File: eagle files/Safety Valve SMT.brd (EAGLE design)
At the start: 39.4 x 107.9 mm, 31 parts, among them IC1 TL072

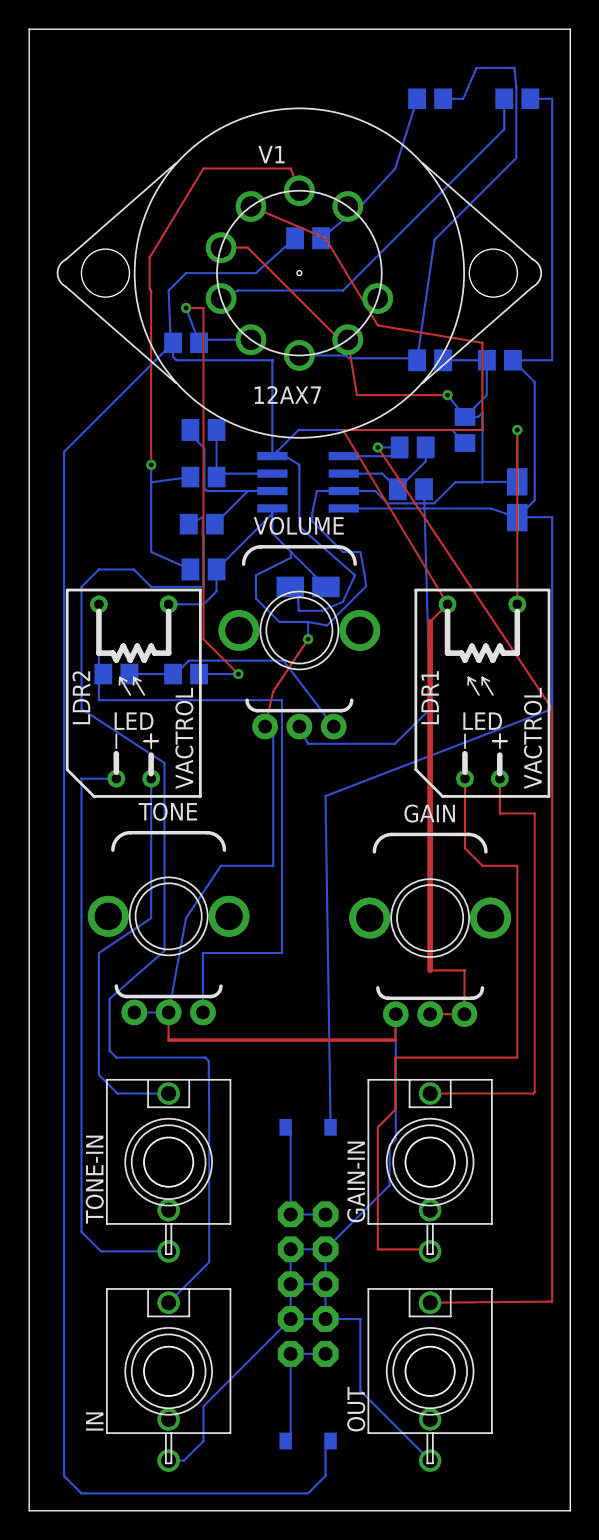
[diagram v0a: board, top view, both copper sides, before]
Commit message: Tidied up a bit
- Mittered traces
- Enlarged the width of them
- fixed two overlapping
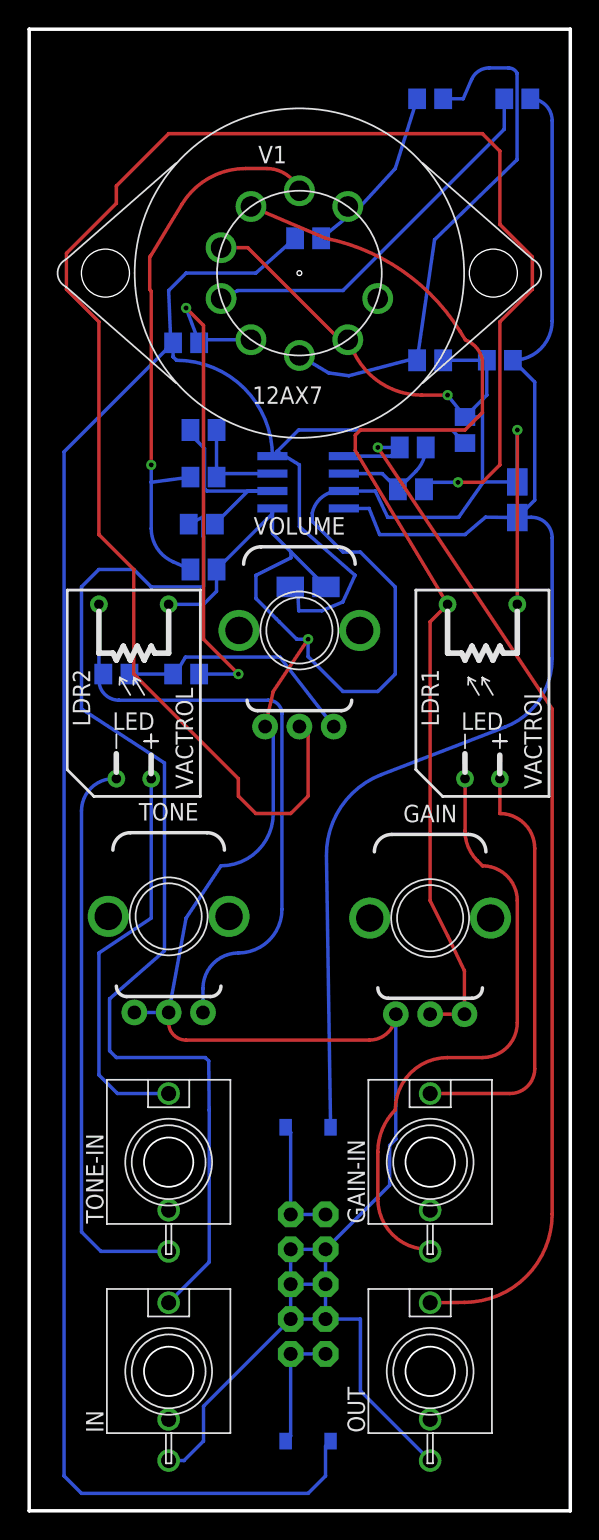
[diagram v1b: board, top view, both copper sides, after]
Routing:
- net N$19: track 27.3 -> 123.7 mm, vias 0 -> 1
- net N$23: track 50.6 -> 42.8 mm
- net N$1: track 88.4 -> 82.5 mm
- net GND: track 240.1 -> 245.4 mm
- net N$17: track 49.2 -> 44.4 mm
- net -12V: track 107.2 -> 102.5 mm
- net +12V: track 173.5 -> 169.3 mm
- net N$4: track 80.9 -> 77.2 mm
- net N$22: track 33.1 -> 30.6 mm
- net N$7: track 43.2 -> 41.2 mm
- net N$21: track 42.5 -> 41.1 mm
- net N$5: track 38.4 -> 37.7 mm
